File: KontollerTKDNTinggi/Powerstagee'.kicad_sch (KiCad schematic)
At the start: 71 parts, among them Q20 HY5110W, Q21 HY5110W, Q22 HY5110W, Q23 HY5110W, Q24 HY5110W, Q25 HY5110W, Q26 HY5110W, Q27 HY5110W, Q28 HY5110W, Q29 HY5110W, Q30 HY5110W, Q31 HY5110W, Q38 HY5110W, Q39 HY5110W, Q40 HY5110W, Q41 HY5110W, Q42 HY5110W, Q43 HY5110W, U5 ACS758xCB-150U-PFF

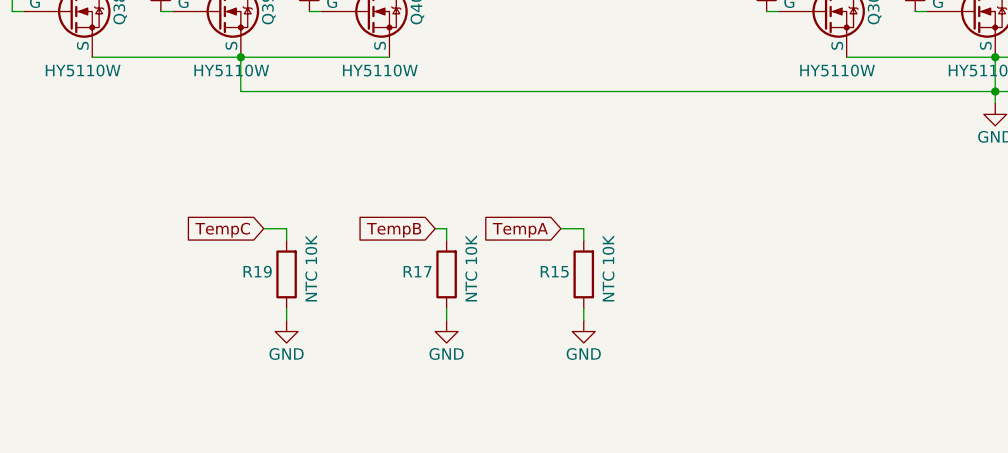
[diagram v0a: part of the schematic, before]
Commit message: mendekatifix
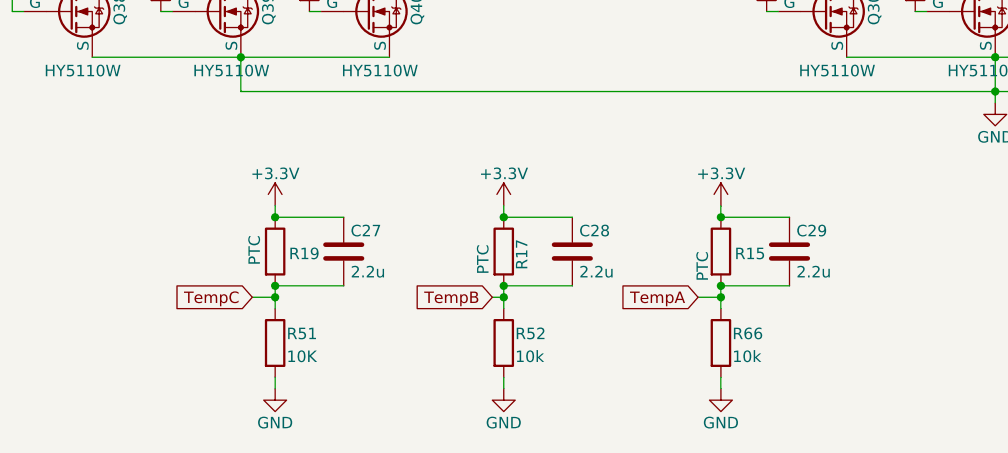
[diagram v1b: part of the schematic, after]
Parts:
- added C27, C28, C29: 2.2u, Capacitor_SMD:C_0805_2012Metric_Pad1.18x1.45mm_HandSolder, symbol Device:C
- added R51: 10K, Resistor_SMD:R_0805_2012Metric_Pad1.20x1.40mm_HandSolder, symbol Device:R
- added R52, R66: 10k, Resistor_SMD:R_0805_2012Metric_Pad1.20x1.40mm_HandSolder, symbol Device:R
- R15, R17, R19: value NTC 10K -> PTC
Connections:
- net +3.3V: now also R15.1, R17.1, R19.1, C27.1, C28.1, C29.1
- net GND: now also R51.2, R52.2, R66.2; no longer R15.1, R17.1, R19.1
- net TempA: now also C29.2, R66.1
- net TempB: now also C28.2, R52.1
- net TempC: now also C27.2, R51.1
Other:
- moved on the sheet: R15, R17, R19
